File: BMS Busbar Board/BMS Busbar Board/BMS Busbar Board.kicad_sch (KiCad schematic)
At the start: 16 parts, among them J1 2005280090

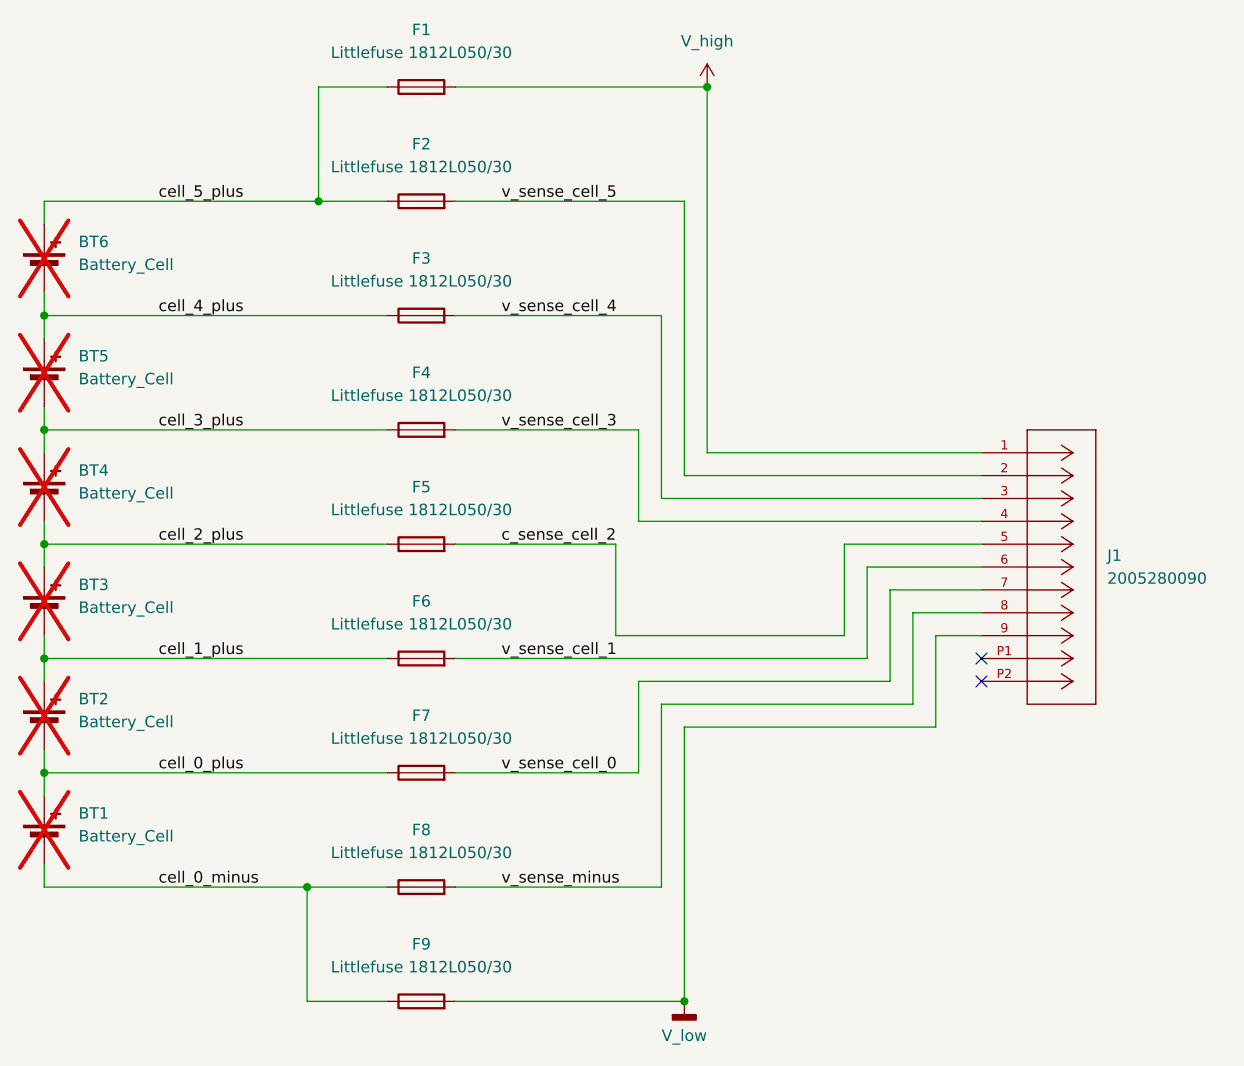
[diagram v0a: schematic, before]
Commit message: changed connector to 5pin version
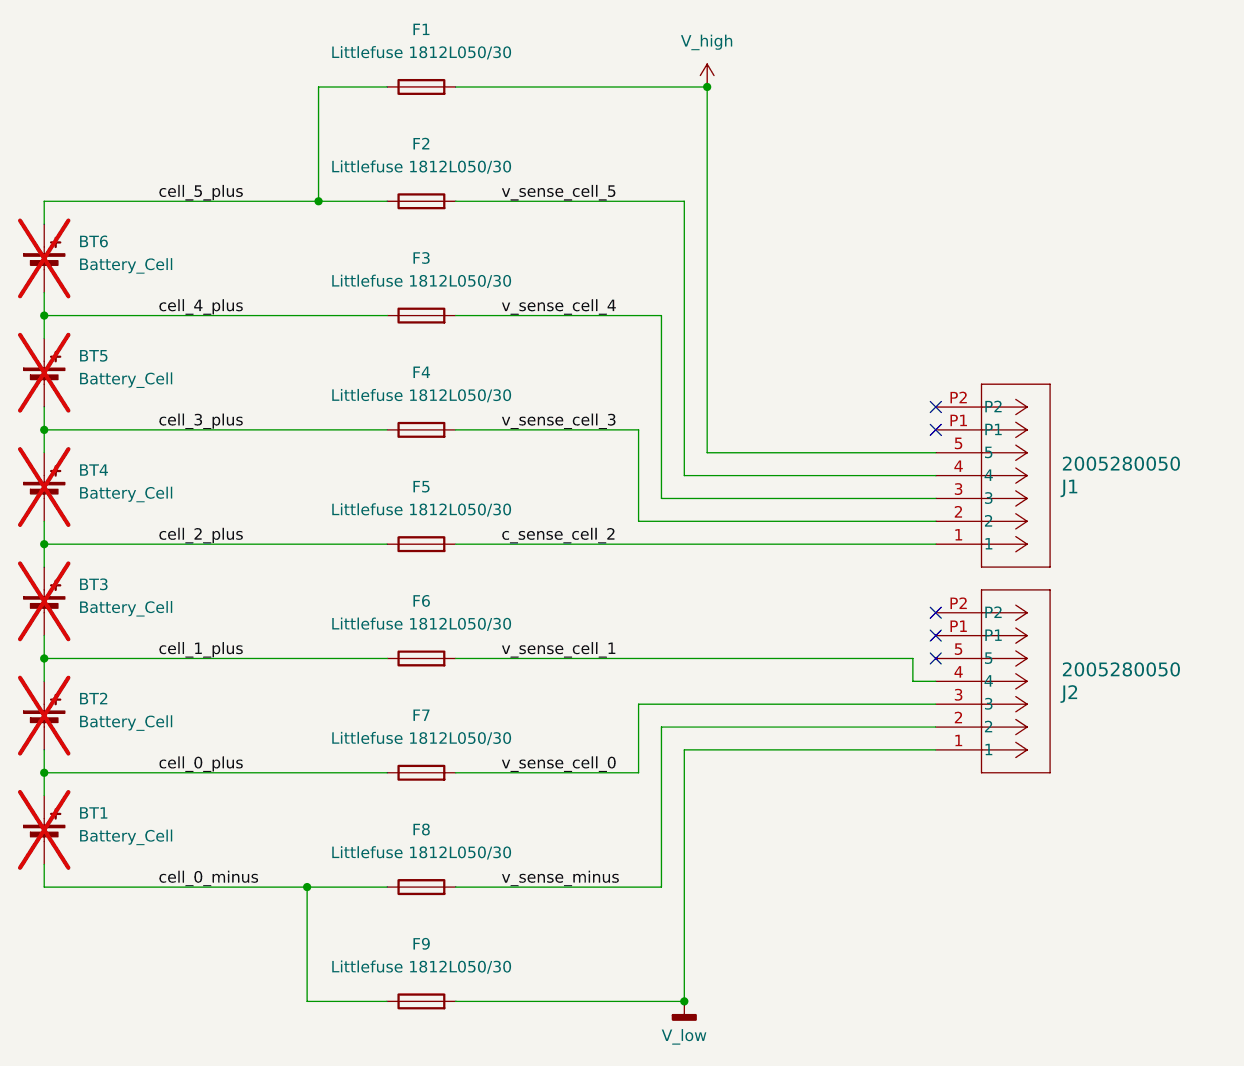
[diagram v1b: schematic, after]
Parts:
- removed J1: 2005280090, FS_4_Global_Footprint_Library:CON_2005280090_MOL, symbol FS_4_Global_Symbol_Library:2005280090
- added J1, J2: 2005280050, FS_4_Global_Footprint_Library:CON_2005280050_MOL, symbol FS_4_Global_Symbol_Library:2005280050
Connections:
- net V_high: now also J1.5
- net V_low: now also J2.1
- net c_sense_cell_2: now also J1.1
- net v_sense_cell_0: now also J2.3
- net v_sense_cell_1: now also J2.4
- net v_sense_cell_3: now also J1.2
- net v_sense_cell_4: now also J1.3
- net v_sense_cell_5: now also J1.4
- net v_sense_minus: now also J2.2
- no-connect marks 2 -> 5
